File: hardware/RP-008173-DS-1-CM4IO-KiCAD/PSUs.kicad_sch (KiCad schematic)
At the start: 33 parts, among them J19 Barrel_Jack, J20 AMP171826-4, Q1 DMP3013SFV-7, U16 AP64501SP-13

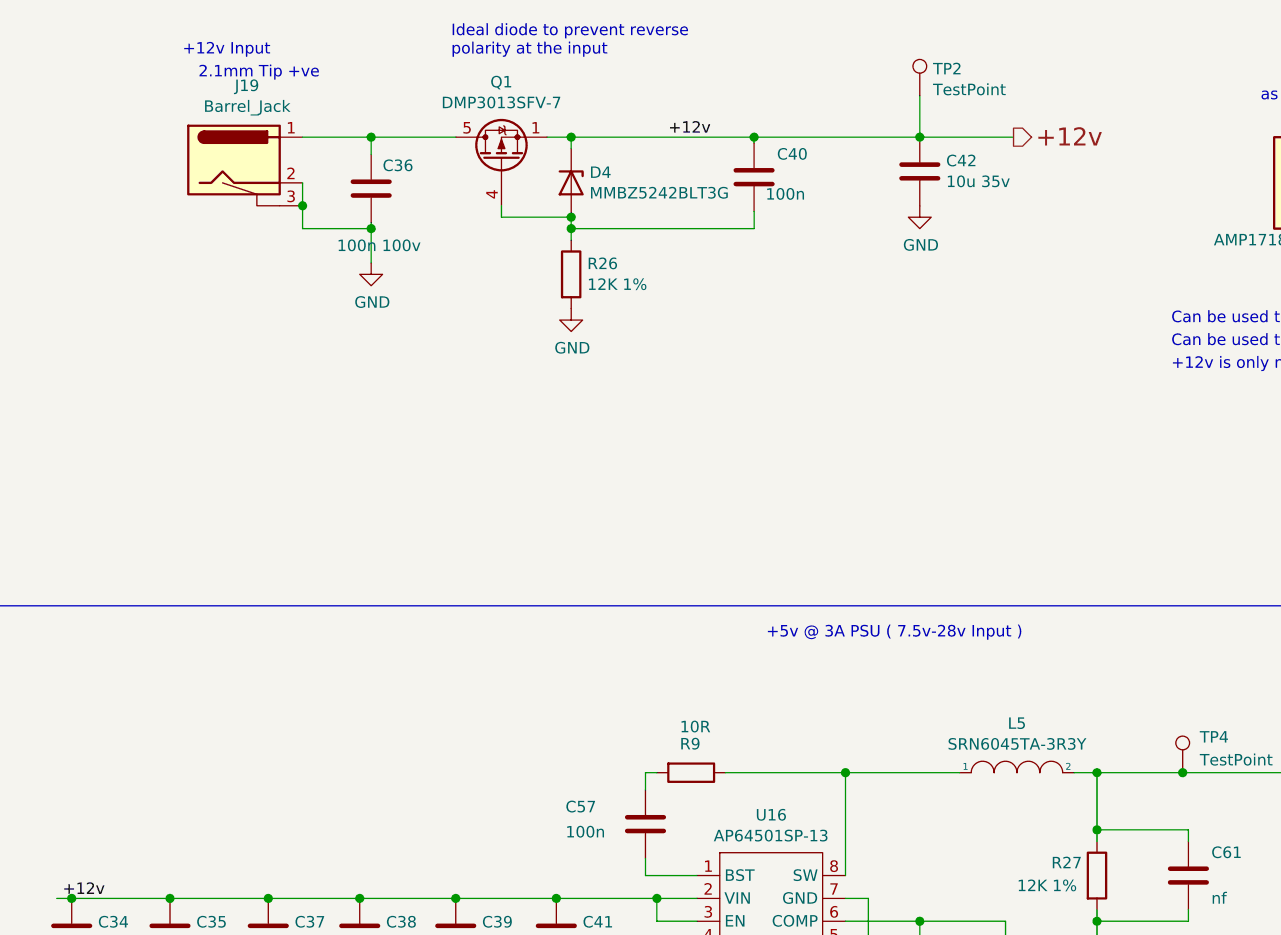
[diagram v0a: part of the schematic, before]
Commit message: added current project
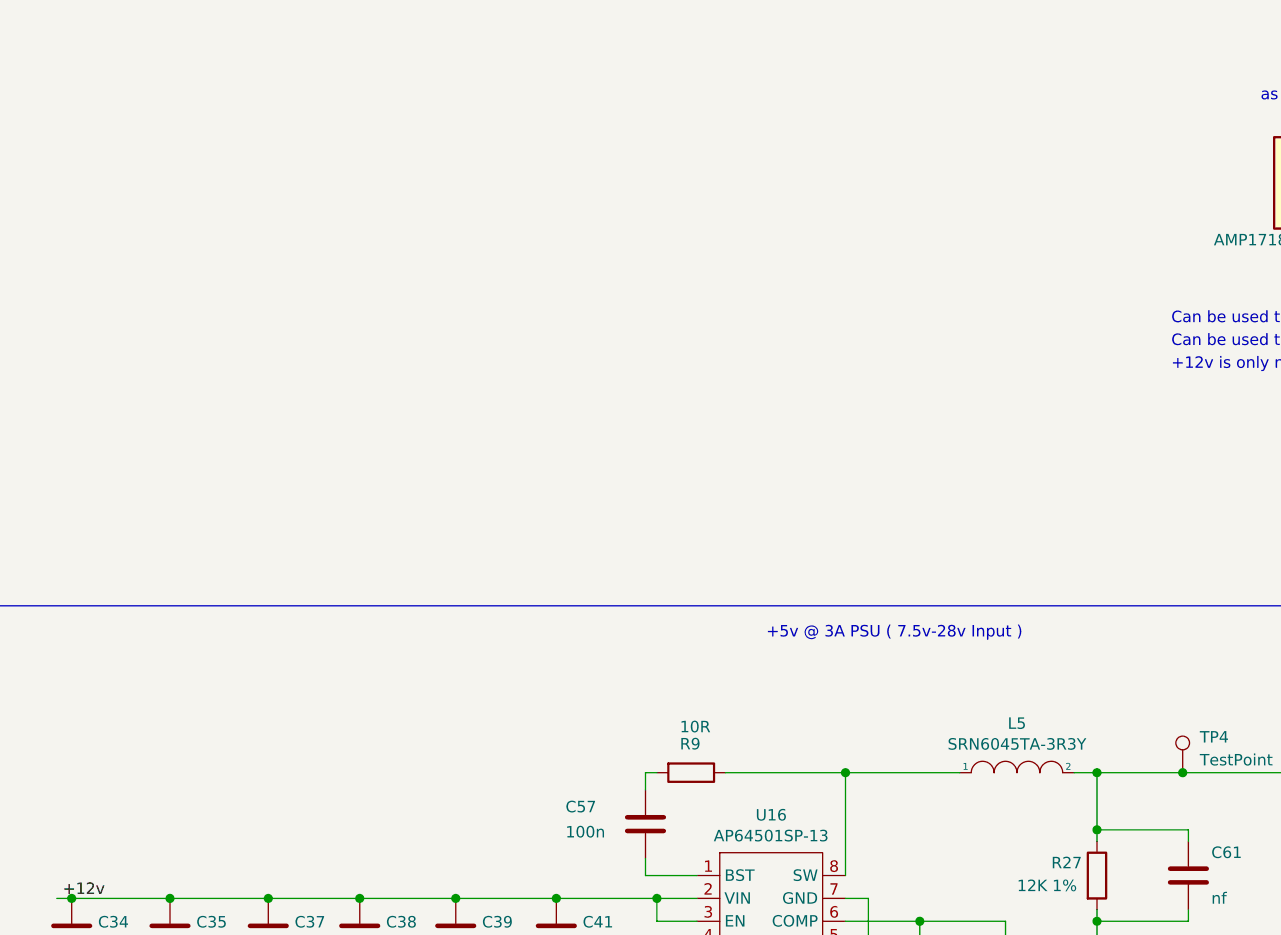
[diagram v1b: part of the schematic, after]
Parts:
- removed C36: 100n 100v, Capacitor_SMD:C_0402_1005Metric, symbol Device:C
- removed C40: 100n, Capacitor_SMD:C_0402_1005Metric, symbol Device:C
- removed C42: 10u 35v, Capacitor_SMD:C_0805_2012Metric, symbol Device:C
- removed D4: MMBZ5242BLT3G, Diode_SMD:D_SOT-23_ANK, symbol Diode:BZX84Cxx
- removed J19: Barrel_Jack, CM4IO:BarrelJack_Horizontal, symbol CM4IO:Barrel_Jack
- removed Q1: DMP3013SFV-7, Package_SON:Diodes_PowerDI3333-8, symbol Transistor_FET:DMP3013SFV
- removed R26: 12K 1%, Resistor_SMD:R_0402_1005Metric, symbol Device:R
- removed TP2: TestPoint, TestPoint:TestPoint_Pad_2.0x2.0mm, symbol Connector:TestPoint
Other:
- note removed: "+12v Input"
- note removed: "2.1mm Tip +ve"
- note removed: "Ideal diode to prevent reverse polarity at the input"
